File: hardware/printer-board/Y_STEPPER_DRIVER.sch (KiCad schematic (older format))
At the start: 9 parts, among them J5 MS_SELECT, J6 Y, U4 A4988_MODULE

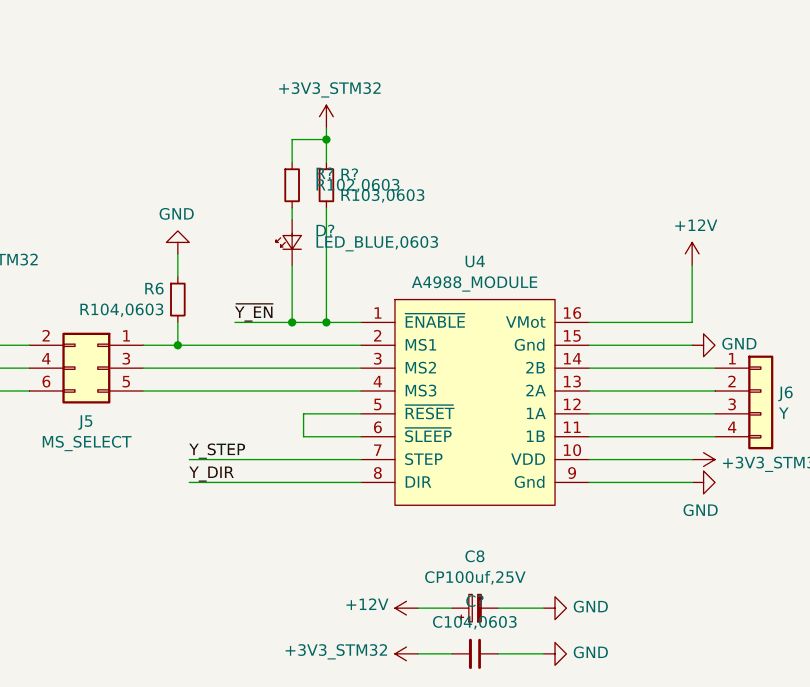
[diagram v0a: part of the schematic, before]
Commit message: update annotations,
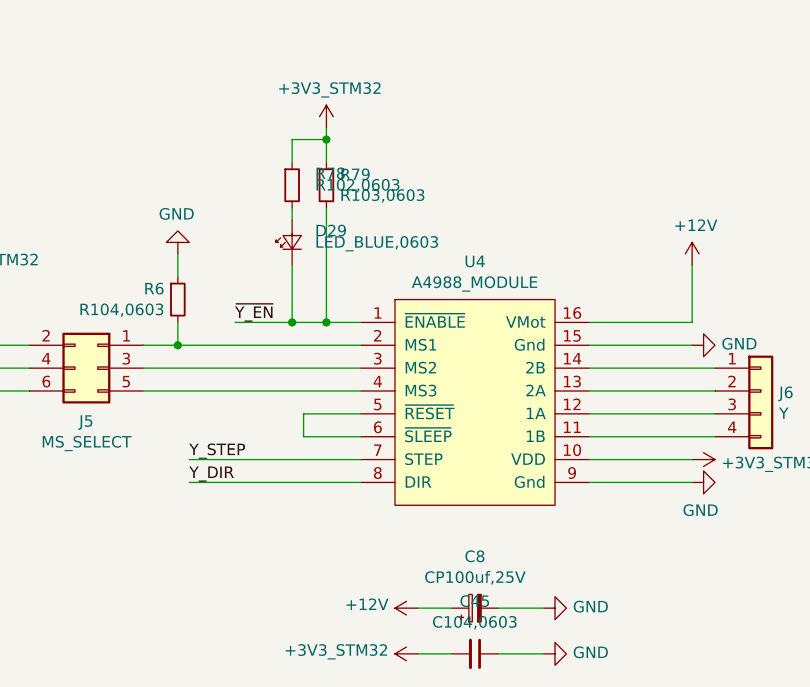
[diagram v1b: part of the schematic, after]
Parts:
- gave numbers to parts that had none: 4
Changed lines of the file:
@@
 $EndBitmap
 $Comp
-L taobao-c:C104,0603 C?
+L taobao-c:C104,0603 C45
 U 1 1 5CC40ACD
 P 5650 4250
-F 0 "C?" V 5421 4250 50  0000 C CNN
+F 0 "C45" V 5421 4250 50  0000 C CNN
 F 1 "C104,0603" V 5512 4250 50  0000 C CNN
 F 2 "Capacitor_SMD:C_0603_1608Metric_Pad1.05x0.95mm_HandSolder" H 5650 4250 50  0001 C CNN
@@
 $EndComp
 $Comp
-L taobao-components:+3V3_STM32 #PWR?
+L taobao-components:+3V3_STM32 #PWR095
 U 1 1 5CC40CD3
 P 3500 2700
-F 0 "#PWR?" H 3500 2550 50  0001 C CNN
+F 0 "#PWR095" H 3500 2550 50  0001 C CNN
 F 1 "+3V3_STM32" H 3515 2873 50  0000 C CNN
 F 2 "" H 3500 2700 50  0001 C CNN
@@
 $EndComp
 $Comp
-L taobao-components:+3V3_STM32 #PWR?
+L taobao-components:+3V3_STM32 #PWR097
 U 1 1 5CC40CEC
 P 5400 4250
-F 0 "#PWR?" H 5400 4100 50  0001 C CNN
+F 0 "#PWR097" H 5400 4100 50  0001 C CNN
 F 1 "+3V3_STM32" V 5415 4378 50  0000 L CNN
 F 2 "" H 5400 4250 50  0001 C CNN
@@
 $EndComp
 $Comp
-L taobao-components:+3V3_STM32 #PWR?
+L taobao-components:+3V3_STM32 #PWR096
 U 1 1 5CC40D1A
 P 6600 3400
-F 0 "#PWR?" H 6600 3250 50  0001 C CNN
+F 0 "#PWR096" H 6600 3250 50  0001 C CNN
 F 1 "+3V3_STM32" V 6615 3528 50  0000 L CNN
 F 2 "" H 6600 3400 50  0001 C CNN
@@
 AR Path="/5CC02AB8/5CC5FBD8" Ref="R?"  Part="1"
 AR Path="/5CC049BB/5CC5FBD8" Ref="R?"  Part="1"
-AR Path="/5CC0A4B9/5CC5FBD8" Ref="R?"  Part="1"
+AR Path="/5CC0A4B9/5CC5FBD8" Ref="R79"  Part="1"
 AR Path="/5CC0A53C/5CC5FBD8" Ref="R?"  Part="1"
 AR Path="/5CC0A8C5/5CC5FBD8" Ref="R?"  Part="1"
@@
 AR Path="/5CC0A8CF/5CC5FBD8" Ref="R?"  Part="1"
 AR Path="/5CC0AEC9/5CC5FBD8" Ref="R?"  Part="1"
-F 0 "R?" H 5059 2246 50  0000 L CNN
+F 0 "R79" H 5059 2246 50  0000 L CNN
 F 1 "R103,0603" H 5059 2155 50  0000 L CNN
 F 2 "Resistor_SMD:R_0603_1608Metric_Pad1.05x0.95mm_HandSolder" H 5000 2200 50  0001 C CNN
@@
 P 5000 1950
 AR Path="/5CC0AEC9/5CC5FBE0" Ref="#PWR?"  Part="1"
-AR Path="/5CC0A4B9/5CC5FBE0" Ref="#PWR?"  Part="1"
-F 0 "#PWR?" H 5000 1800 50  0001 C CNN
+AR Path="/5CC0A4B9/5CC5FBE0" Ref="#PWR094"  Part="1"
+F 0 "#PWR094" H 5000 1800 50  0001 C CNN
 F 1 "+3V3_STM32" H 5015 2123 50  0000 C CNN
 F 2 "" H 5000 1950 50  0001 C CNN
@@
 AR Path="/5CC15C35/5CC5FBE6" Ref="R?"  Part="1"
 AR Path="/5CC0AEC9/5CC5FBE6" Ref="R?"  Part="1"
-AR Path="/5CC0A4B9/5CC5FBE6" Ref="R?"  Part="1"
-F 0 "R?" H 4950 2250 50  0000 L CNN
+AR Path="/5CC0A4B9/5CC5FBE6" Ref="R78"  Part="1"
+F 0 "R78" H 4950 2250 50  0000 L CNN
 F 1 "R102,0603" H 4950 2200 50  0000 L CNN
 F 2 "Resistor_SMD:R_0603_1608Metric_Pad1.05x0.95mm_HandSolder" H 4850 2200 50  0001 C CNN
@@
 AR Path="/5CC15C35/5CC5FBED" Ref="D?"  Part="1"
 AR Path="/5CC0AEC9/5CC5FBED" Ref="D?"  Part="1"
-AR Path="/5CC0A4B9/5CC5FBED" Ref="D?"  Part="1"
-F 0 "D?" V 4900 2350 50  0000 R CNN
+AR Path="/5CC0A4B9/5CC5FBED" Ref="D29"  Part="1"
+F 0 "D29" V 4900 2350 50  0000 R CNN
 F 1 "LED_BLUE,0603" V 4850 2350 50  0000 R CNN
 F 2 "LED_SMD:LED_0603_1608Metric_Pad1.05x0.95mm_HandSolder" V 4850 2450 50  0001 C CNN
